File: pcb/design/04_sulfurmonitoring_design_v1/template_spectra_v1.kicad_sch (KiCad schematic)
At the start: 14 parts, among them U1 Heltec_WSL_V3, U2 Anemometer, U3 Micro_SDCARD_v2, U4 Wind_Direction, U5 W5500_Module, U6 BUCK_MP1584_3V3

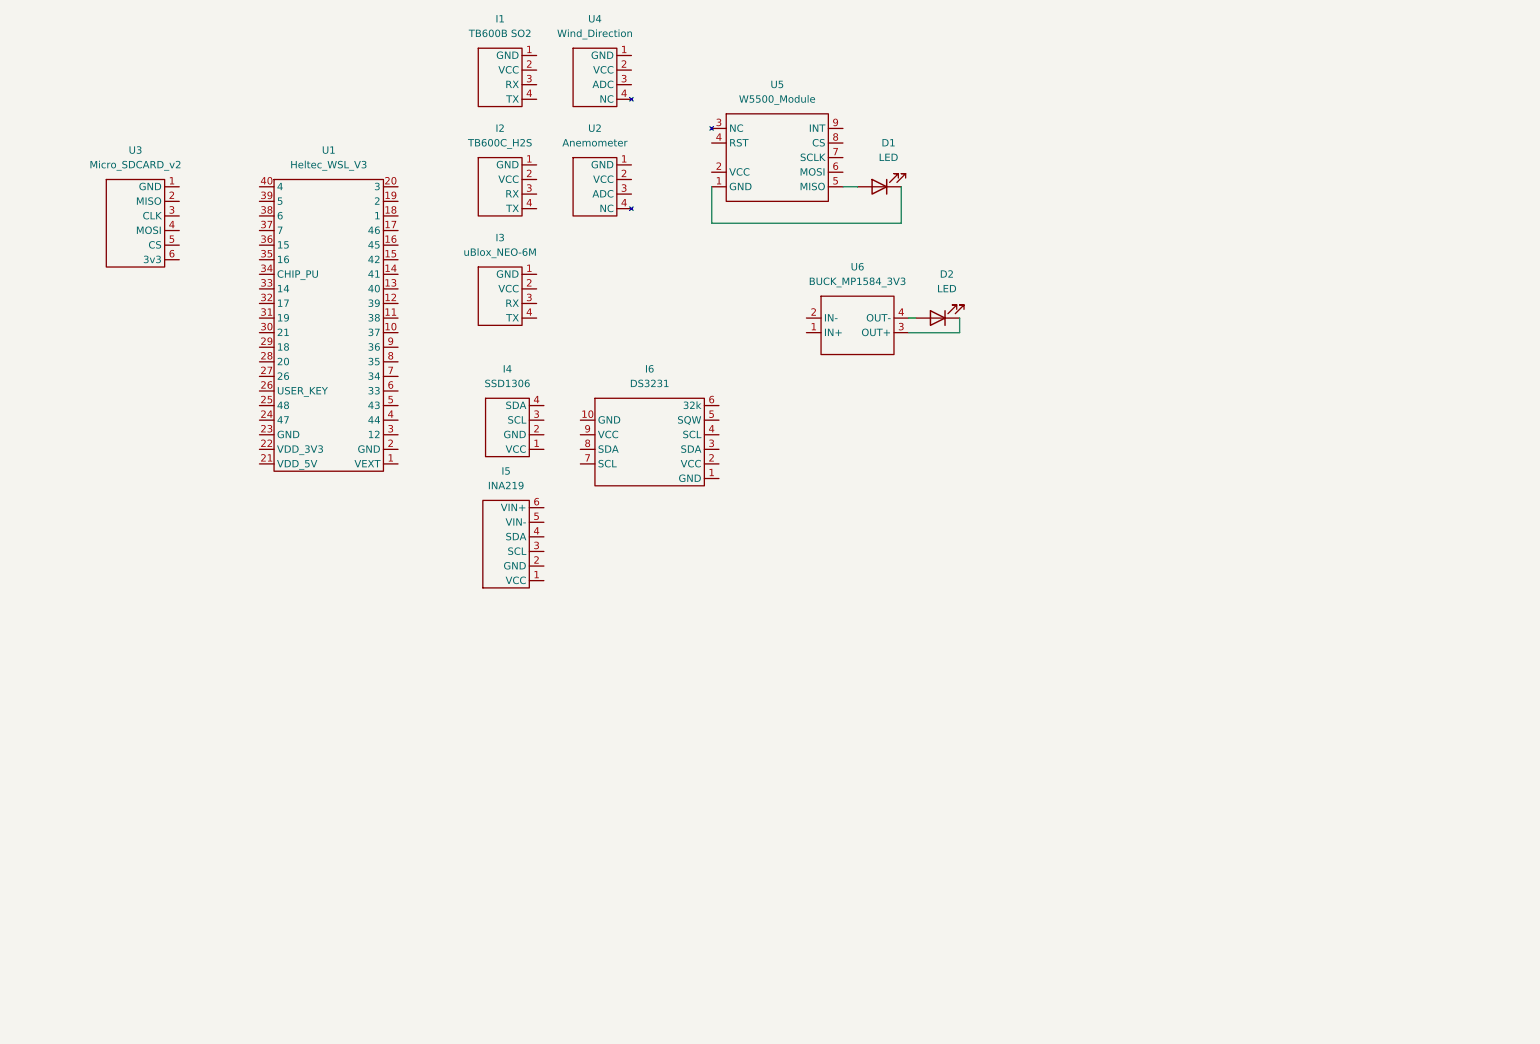
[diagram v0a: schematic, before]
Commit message: update design
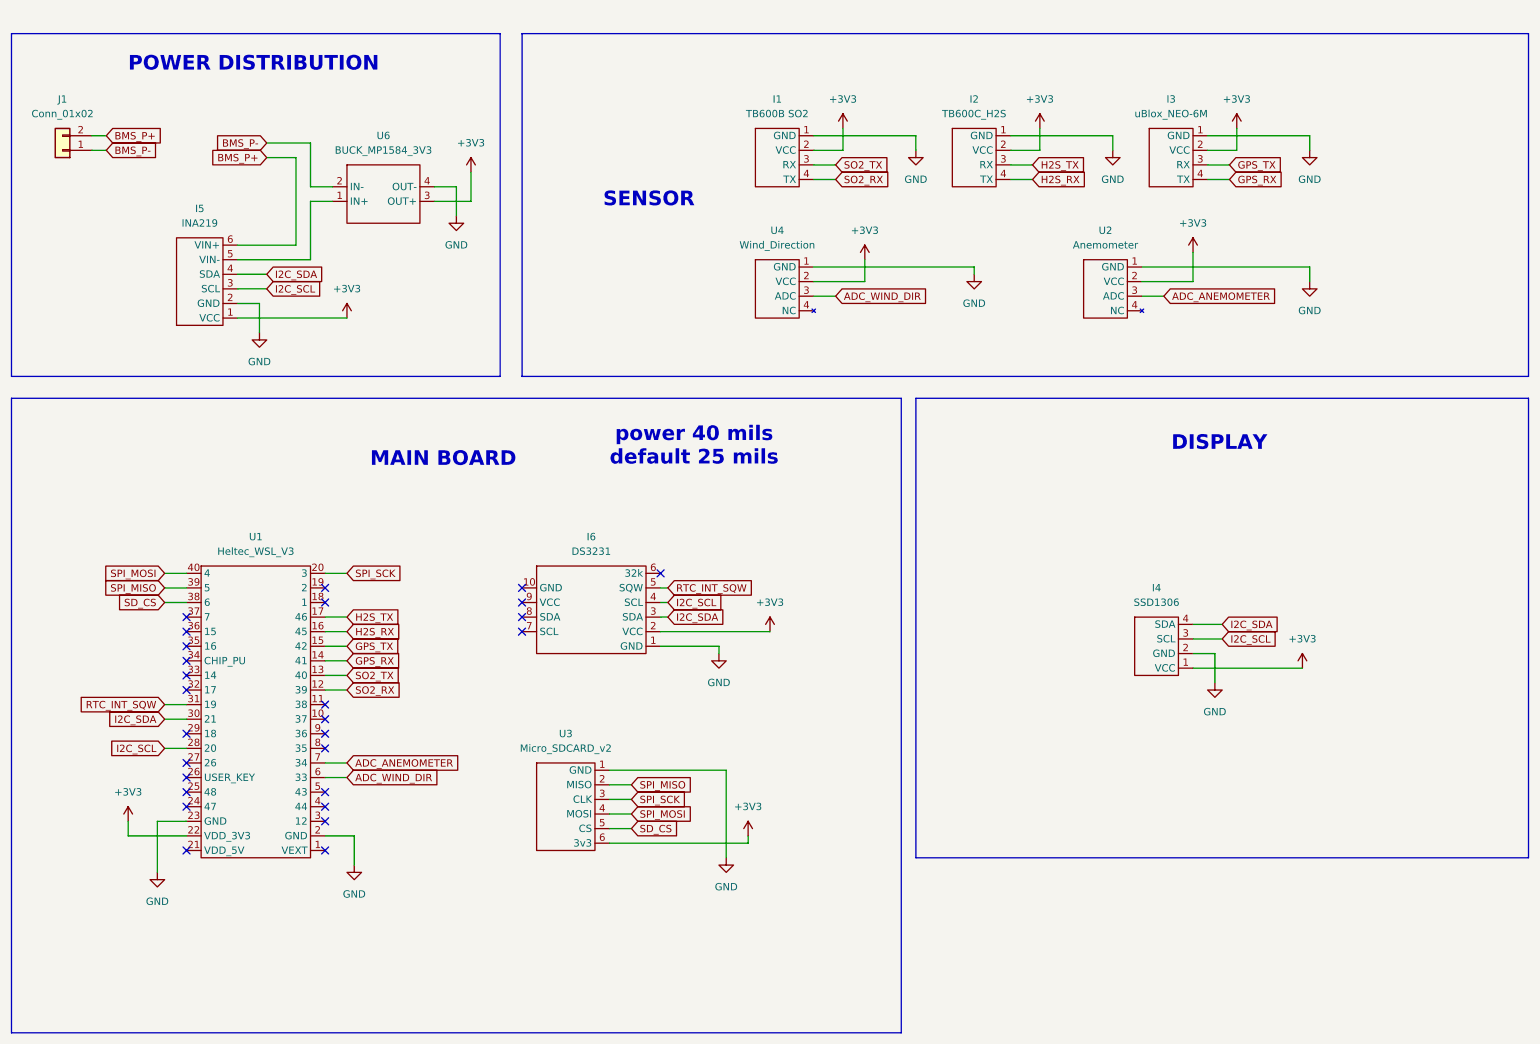
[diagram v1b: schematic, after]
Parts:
- removed D1, D2: LED, LED_THT:LED_D5.0mm, symbol Device:LED
- removed U5: W5500_Module, Custom Board:W5500_Module, symbol Custom Board:w5500_module
- added J1: Conn_01x02, Connector_JST:JST_XH_B2B-XH-A_1x02_P2.50mm_Vertical, symbol Connector_Generic:Conn_01x02
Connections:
- net GND: now reaches U4.1 (GND)
- net GND: now also I1.1 (GND), I2.1 (GND), I3.1 (GND), I4.2 (GND), I5.2 (GND), I6.1 (GND), U1.2 (GND), U1.23 (GND), U2.1 (GND), U3.1 (GND), U6.4 (OUT-)
- net +3V3: now reaches U4.2 (VCC)
- net +3V3: now also I1.2 (VCC), I2.2 (VCC), I3.2 (VCC), I4.1 (VCC), I5.1 (VCC), I6.2 (VCC), U1.22 (VDD_3V3), U2.2 (VCC), U3.6 (3v3), U6.3 (OUT+)
- net ADC_WIND_DIR: now reaches U4.3 (ADC)
- net ADC_WIND_DIR: now also U1.6 (33)
- net SO2_TX: now reaches I1.3 (RX)
- net SO2_TX: now also U1.13 (40)
- net SO2_RX: now reaches I1.4 (TX)
- net SO2_RX: now also U1.12 (39)
- net GPS_TX: now reaches I3.3 (RX)
- net GPS_TX: now also U1.15 (42)
- net GPS_RX: now reaches I3.4 (TX)
- net GPS_RX: now also U1.14 (41)
- net ADC_ANEMOMETER: now reaches U2.3 (ADC)
- net ADC_ANEMOMETER: now also U1.7 (34)
- net I2C_SDA: now reaches I6.3 (SDA)
- net I2C_SDA: now also I4.4 (SDA), I5.4 (SDA), U1.30 (21)
- net I2C_SCL: now reaches I6.4 (SCL)
- net I2C_SCL: now also I4.3 (SCL), I5.3 (SCL), U1.28 (20)
- net RTC_INT_SQW: now reaches I6.5 (SQW)
- net RTC_INT_SQW: now also U1.31 (19)
- net SPI_MISO: now reaches U3.2 (MISO)
- net SPI_MISO: now also U1.39 (5)
- net SPI_SCK: now reaches U3.3 (CLK)
- net SPI_SCK: now also U1.20 (3)
- net SPI_MOSI: now reaches U3.4 (MOSI)
- net SPI_MOSI: now also U1.40 (4)
- net SD_CS: now reaches U3.5 (CS)
- net SD_CS: now also U1.38 (6)
- net at I5.5 (VIN-): now also U6.1 (IN+)
- net BMS_P+: now reaches I5.6 (VIN+)
- net BMS_P+: now also J1.2 (Pin_2)
- net H2S_TX: now reaches I2.3 (RX)
- net H2S_TX: now also U1.17 (46)
- net H2S_RX: now reaches I2.4 (TX)
- net H2S_RX: now also U1.16 (45)
- net BMS_P-: now reaches U6.2 (IN-)
- net BMS_P-: now also J1.1 (Pin_1)
- no-connect marks 0 -> 27
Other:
- note added: "DISPLAY"
- note added: "MAIN BOARD"
- note added: "POWER DISTRIBUTION"
- note added: "SENSOR"
- note added: "power 40 mils default 25 mils"
- moved on the sheet: I1, I2, I3, I4, I5, I6, U1, U2, U3, U4, U6

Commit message: update design
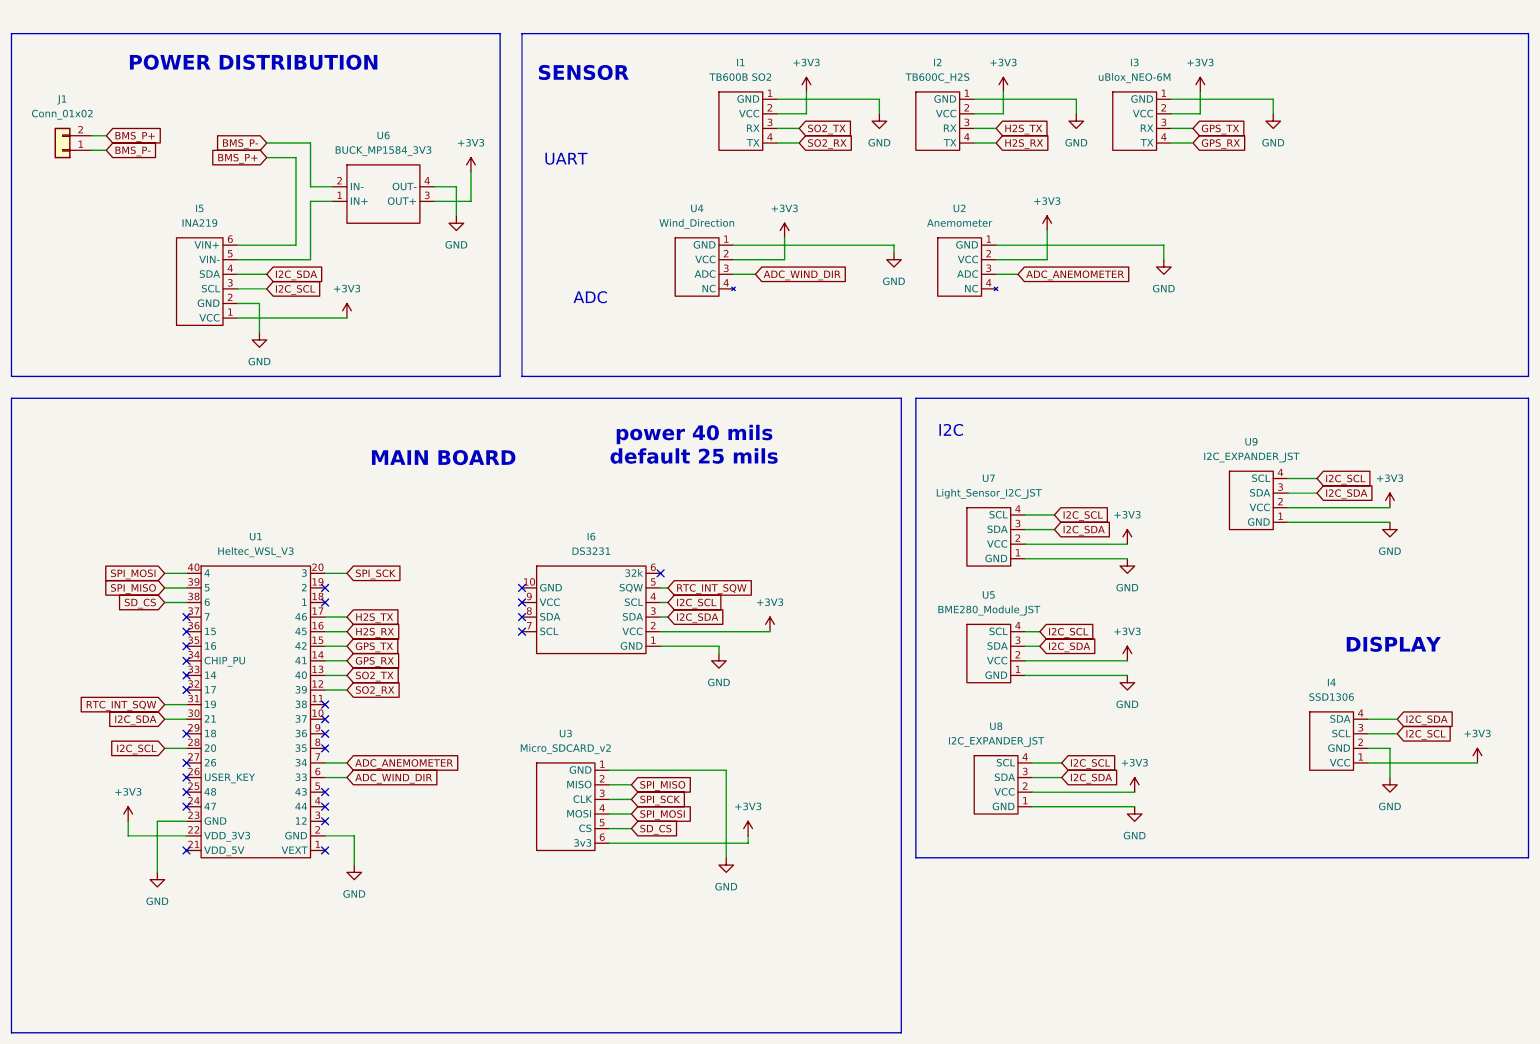
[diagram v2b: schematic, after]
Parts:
- added U5: BME280_Module_JST, Connector_JST:JST_XH_B4B-XH-A_1x04_P2.50mm_Vertical, symbol Custom Board:BME280_Module_JST
- added U7: Light_Sensor_I2C_JST, Connector_JST:JST_XH_B4B-XH-A_1x04_P2.50mm_Vertical, symbol Custom Board:Light_Sensor_I2C_JST
- added U8, U9: I2C_EXPANDER_JST, Connector_JST:JST_XH_B4B-XH-A_1x04_P2.50mm_Vertical, symbol Custom Board:I2C_EXPANDER_JST
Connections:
- net +3V3: now also U5.2 (VCC), U7.2 (VCC), U8.2 (VCC), U9.2 (VCC)
- net GND: now also U5.1 (GND), U7.1 (GND), U8.1 (GND), U9.1 (GND)
- net I2C_SCL: now also U5.4 (SCL), U7.4 (SCL), U8.4 (SCL), U9.4 (SCL)
- net I2C_SDA: now also U5.3 (SDA), U7.3 (SDA), U8.3 (SDA), U9.3 (SDA)
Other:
- note added: "ADC"
- note added: "I2C"
- note added: "UART"
- moved on the sheet: I1, I2, I3, I4, U2, U4

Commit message: update drc
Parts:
- I1: footprint Custom Board:TB600B_SO2 -> Custom Board:TB600B_SO2_Module
- I2: footprint Custom Board:TB600C_H2S -> Custom Board:TB600C_H2S_Module
- I3: footprint Custom Board:uBlox_NEO-6M_JST -> Custom Board:uBlox_NEO-6M_Module_JST
- I4: footprint Custom Board:SSD1306_onBoard -> Custom Board:SSD1306_Module
- I5: footprint Custom Board:INA219 -> Custom Board:INA219_Module
- I6: footprint Custom Board:DS3231 -> Custom Board:DS3231_Module
- U1: footprint Custom Board:Heltec_WSL_V3_v1 -> Custom Board:Heltec_WSL_V3_Module
- U2: footprint Custom Board:STASRG_Anemometer -> Custom Board:STASRG_Anemometer_Module
- U3: footprint Custom Board:Micro_SDCARD_v2 -> Custom Board:Micro_SDCARD_v2_Module
- U4: footprint Custom Board:STASRG_Wind_Dir -> Custom Board:STASRG_Wind_Dir_Module
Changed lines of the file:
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@@
 			)
 		)
-		(property "Footprint" "Custom Board:STASRG_Wind_Dir"
+		(property "Footprint" "Custom Board:STASRG_Wind_Dir_Module"
 			(at 136.144 41.148 0)
 			(effects
@@
 			)
 		)
-		(property "Footprint" "Custom Board:TB600B_SO2"
+		(property "Footprint" "Custom Board:TB600B_SO2_Module"
 			(at 143.51 17.018 0)
 			(effects
@@
 			)
 		)
-		(property "Footprint" "Custom Board:uBlox_NEO-6M_JST"
+		(property "Footprint" "Custom Board:uBlox_NEO-6M_Module_JST"
 			(at 212.09 15.748 0)
 			(effects
@@
 			)
 		)
-		(property "Footprint" "Custom Board:STASRG_Anemometer"
+		(property "Footprint" "Custom Board:STASRG_Anemometer_Module"
 			(at 181.61 42.926 0)
 			(effects
@@
 			)
 		)
-		(property "Footprint" "Custom Board:DS3231"
+		(property "Footprint" "Custom Board:DS3231_Module"
 			(at 116.84 100.838 0)
 			(effects
@@
 			)
 		)
-		(property "Footprint" "Custom Board:Micro_SDCARD_v2"
+		(property "Footprint" "Custom Board:Micro_SDCARD_v2_Module"
 			(at 113.03 137.668 0)
 			(effects
@@
 			)
 		)
-		(property "Footprint" "Custom Board:INA219"
+		(property "Footprint" "Custom Board:INA219_Module"
 			(at 49.784 44.196 0)
 			(effects
@@
 			)
 		)
-		(property "Footprint" "Custom Board:TB600C_H2S"
+		(property "Footprint" "Custom Board:TB600C_H2S_Module"
 			(at 179.07 16.002 0)
 			(effects
@@
 			)
 		)
-		(property "Footprint" "Custom Board:Heltec_WSL_V3_v1"
+		(property "Footprint" "Custom Board:Heltec_WSL_V3_Module"
 			(at 58.928 101.092 0)
 			(effects
@@
 			)
 		)
-		(property "Footprint" "Custom Board:SSD1306_onBoard"
+		(property "Footprint" "Custom Board:SSD1306_Module"
 			(at 245.872 124.968 0)
 			(effects
